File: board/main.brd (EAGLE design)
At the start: 37.8 x 39.4 mm, 11 parts, among them Q1 12MHz, U1 ATMEGA328P_TQFP

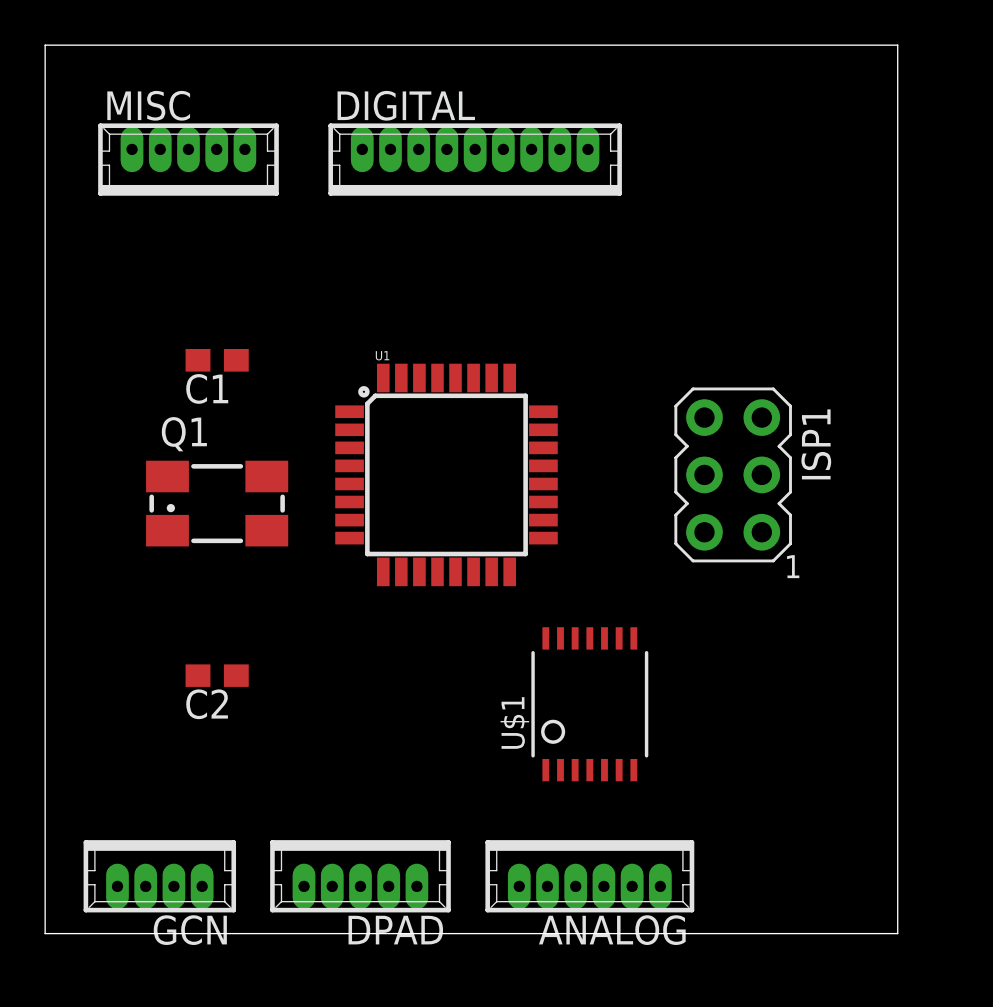
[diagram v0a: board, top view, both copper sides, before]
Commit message: Finished routing
Signed-off-by: Garrett Greenwood <garrettagreenwood@gmail.com>
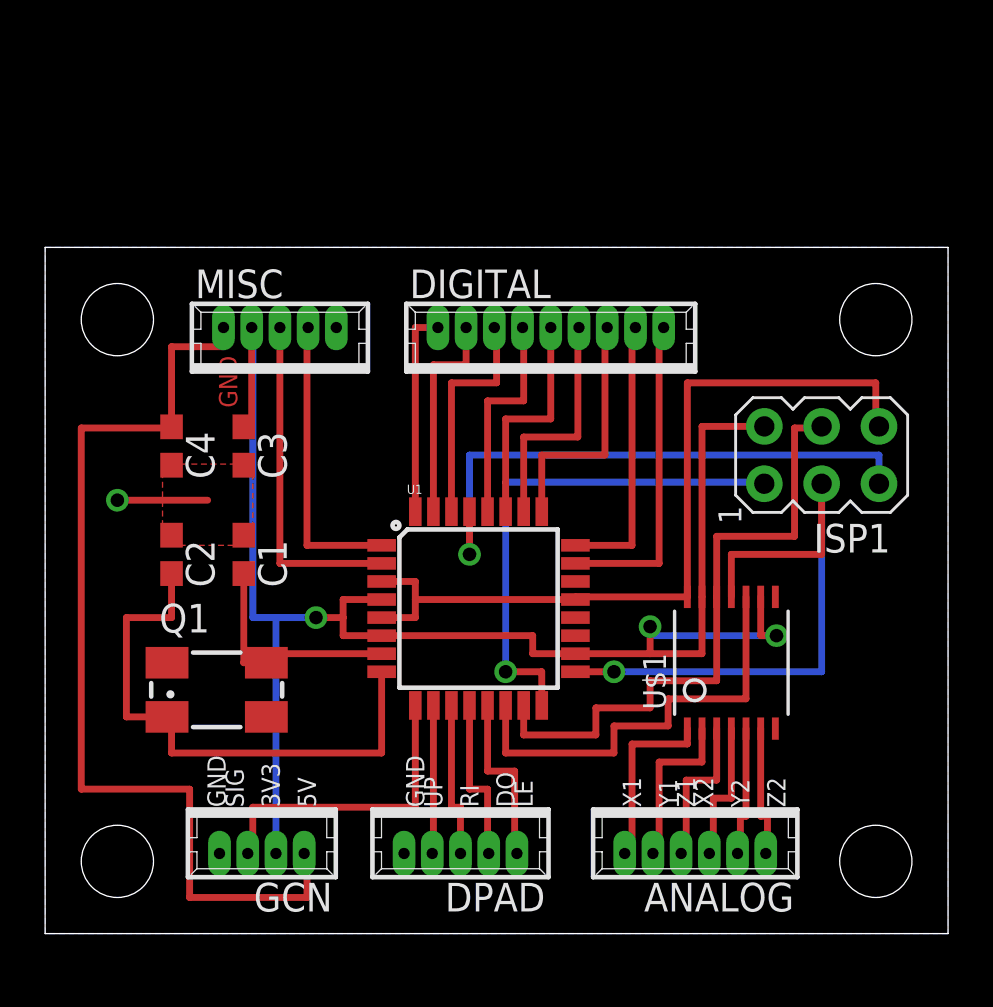
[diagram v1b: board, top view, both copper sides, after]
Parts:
- added C3, C4: .1uF, resistor:C0603
- moved MISC 8.87 mm to (10.4, 26.4)
- moved C1 8.68 mm to (8.80, 16.8), turned to 270 degrees
- moved DIGITAL 8.57 mm to (22.4, 26.4)
- moved Q1 8.25 mm to (7.60, 10.8)
- moved U$1 6.53 mm to (30.4, 12.0)
- moved U1 6.09 mm to (19.2, 14.4)
- moved C2 5.74 mm to (5.60, 16.8), turned to 270 degrees
- moved ANALOG 4.89 mm to (28.8, 4.00)
- moved GCN 4.75 mm to (9.60, 4.00)
- moved DPAD 4.66 mm to (18.4, 4.00)
- moved ISP1 4.02 mm to (34.4, 21.2), turned to 90 degrees
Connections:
- net 3V3: now also C3.1
- net 5V: now also C4.1
- net GND: now also C3.2, C4.2, MISC.1, U1.21
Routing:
- net 3V3: track 0.00 -> 74.6 mm, vias 0 -> 3
- net 5V: track 0.00 -> 43.6 mm
- net GND: track 0.00 -> 40.7 mm, vias 0 -> 1
- net SCK: track 0.00 -> 28.2 mm, vias 0 -> 1
- net MOSI: track 0.00 -> 28.2 mm
- net AVR_RESET: track 0.00 -> 25.7 mm, vias 0 -> 1
- net N$2: track 0.00 -> 24.9 mm
- net N$4: track 0.00 -> 23.0 mm, vias 0 -> 1
- net SS: track 0.00 -> 19.7 mm
- net N$19: track 0.00 -> 15.0 mm
- net N$5: track 0.00 -> 14.4 mm
- net N$18: track 0.00 -> 14.0 mm
- net N$20: track 0.00 -> 13.0 mm
- net N$6: track 0.00 -> 12.3 mm
- net N$7: track 0.00 -> 11.1 mm
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- added copper zone on layer 1, net GND
- added copper zone on layer 16, net GND
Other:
- board size 37.8 x 39.4 mm -> 40 x 30.4 mm
- board text added: "3V3"
- board text added: "5V"
- board text added: "DO"
- board text added: "GND"
- board text added: "LE"
- board text added: "RI"
- board text added: "SIG"
- board text added: "UP"
- board text added: "X1"
- board text added: "X2"
- board text added: "Y1"
- board text added: "Y2"
- board text added: "Z1"
- board text added: "Z2"
